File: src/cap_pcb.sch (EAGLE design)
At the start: 10 parts, among them CON1 PINHEAD_2X02-PTH-2-MALE, CON2 PINHEAD_2X02-PTH-2-MALE, CON3 PINHEAD_2X02-PTH-2-MALE, CON4 PINHEAD_2X02-PTH-2-MALE

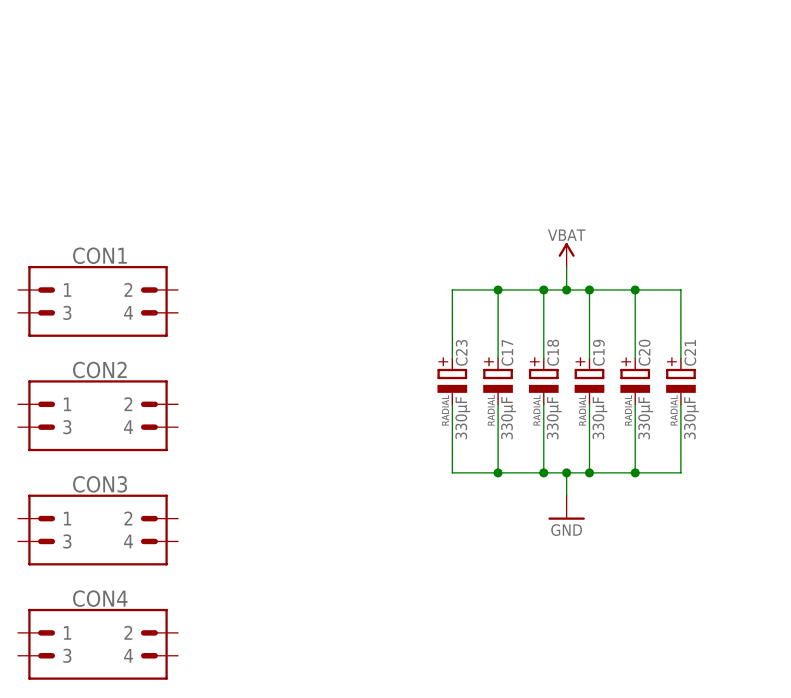
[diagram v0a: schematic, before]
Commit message: capacitor PCB polygons update
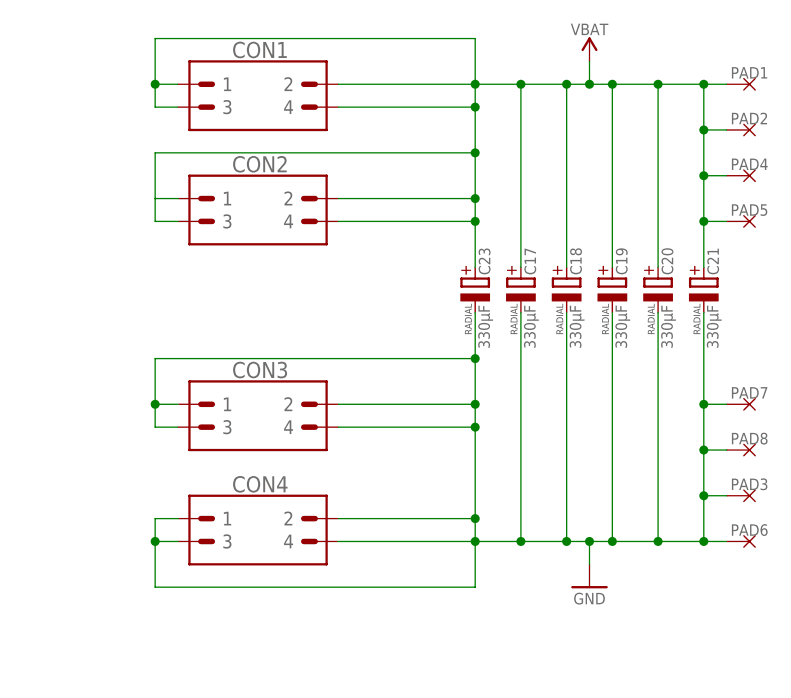
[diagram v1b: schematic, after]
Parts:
- added PAD1, PAD2, PAD3, PAD4, PAD5, PAD6, PAD7, PAD8: PAD-5X4, PADS:PAD-5X4
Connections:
- net GND: now also CON3.1, CON3.2, CON3.3, CON3.4, CON4.1, CON4.2, CON4.3, CON4.4, PAD3.P$1, PAD6.P$1, PAD7.P$1, PAD8.P$1
- net VBAT: now also CON1.1, CON1.2, CON1.3, CON1.4, CON2.1, CON2.2, CON2.3, CON2.4, PAD1.P$1, PAD2.P$1, PAD4.P$1, PAD5.P$1
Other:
- moved on the sheet: C17, C18, C19, C20, C21, C23, CON1, CON2, CON3, CON4

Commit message: Massive routing update
InterPCB connectors between Cap PCB and power PCB replaced with bigger ones
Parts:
- CON1, CON2, CON3, CON4: value PINHEAD_2X02-PTH-2-MALE -> PINHEAD_2X02-PTH-2.54-MALE; device pinhead:PINHEAD_2X02-PTH-2-MALE -> pinhead:PINHEAD_2X02-PTH-2.54-MALE
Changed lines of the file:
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@@
 <part name="+P3" library="supply_symbols" library_urn="urn:adsk.eagle:library:5017758" deviceset="VBAT" device=""/>
 <part name="FRAME1" library="frames" library_urn="urn:adsk.eagle:library:229" deviceset="A5L-LOC" device=""/>
-<part name="CON3" library="pinhead" library_urn="urn:adsk.eagle:library:2540341" deviceset="PINHEAD_2X02" device="-PTH-2-MALE" package3d_urn="urn:adsk.eagle:package:23506355/2">
+<part name="CON3" library="pinhead" library_urn="urn:adsk.eagle:library:2540341" deviceset="PINHEAD_2X02" device="-PTH-2.54-MALE" package3d_urn="urn:adsk.eagle:package:24957333/1" value="PINHEAD_2X02-PTH-2.54-MALE">
 <variant name="basic" populate="no"/>
 </part>
-<part name="CON1" library="pinhead" library_urn="urn:adsk.eagle:library:2540341" deviceset="PINHEAD_2X02" device="-PTH-2-MALE" package3d_urn="urn:adsk.eagle:package:23506355/2"/>
-<part name="CON2" library="pinhead" library_urn="urn:adsk.eagle:library:2540341" deviceset="PINHEAD_2X02" device="-PTH-2-MALE" package3d_urn="urn:adsk.eagle:package:23506355/2"/>
-<part name="CON4" library="pinhead" library_urn="urn:adsk.eagle:library:2540341" deviceset="PINHEAD_2X02" device="-PTH-2-MALE" package3d_urn="urn:adsk.eagle:package:23506355/2"/>
+<part name="CON1" library="pinhead" library_urn="urn:adsk.eagle:library:2540341" deviceset="PINHEAD_2X02" device="-PTH-2.54-MALE" package3d_urn="urn:adsk.eagle:package:24957333/1" value="PINHEAD_2X02-PTH-2.54-MALE"/>
+<part name="CON2" library="pinhead" library_urn="urn:adsk.eagle:library:2540341" deviceset="PINHEAD_2X02" device="-PTH-2.54-MALE" package3d_urn="urn:adsk.eagle:package:24957333/1" value="PINHEAD_2X02-PTH-2.54-MALE"/>
+<part name="CON4" library="pinhead" library_urn="urn:adsk.eagle:library:2540341" deviceset="PINHEAD_2X02" device="-PTH-2.54-MALE" package3d_urn="urn:adsk.eagle:package:24957333/1" value="PINHEAD_2X02-PTH-2.54-MALE"/>
 <part name="PAD4" library="PADS" library_urn="urn:adsk.eagle:library:3188696" deviceset="PAD" device="-5X4" package3d_urn="urn:adsk.eagle:package:5210040/1" value="PAD-5X4">
 <variant name="basic" populate="no"/>
